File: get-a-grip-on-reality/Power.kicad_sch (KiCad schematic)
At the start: 3 parts, among them J1 Battery Connector, U1 BQ25170DSGR, U2 TLV76733DRVx

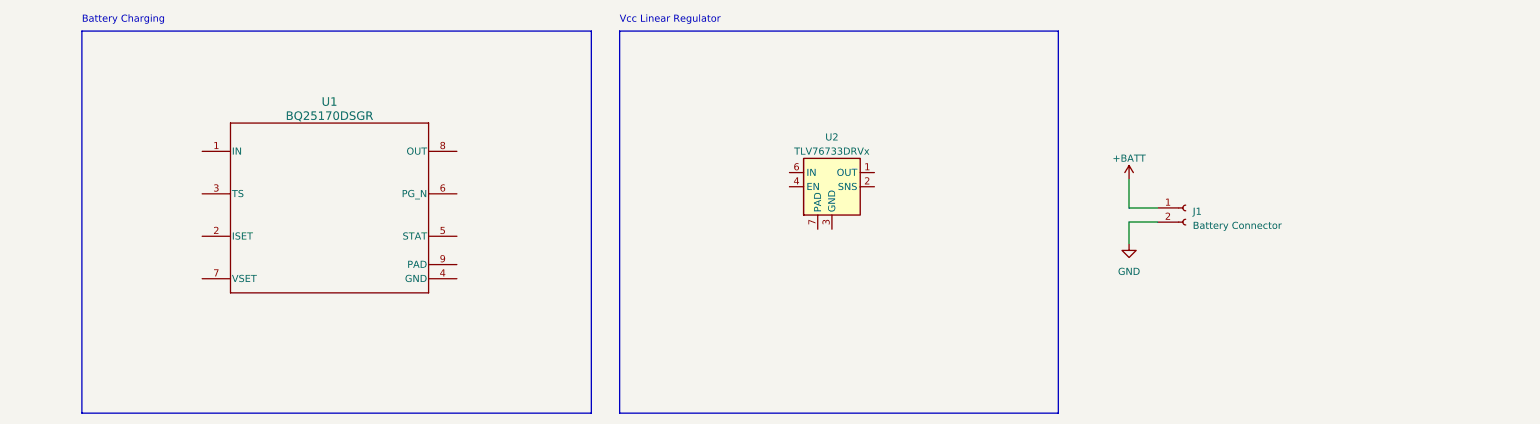
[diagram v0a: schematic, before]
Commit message: power wip
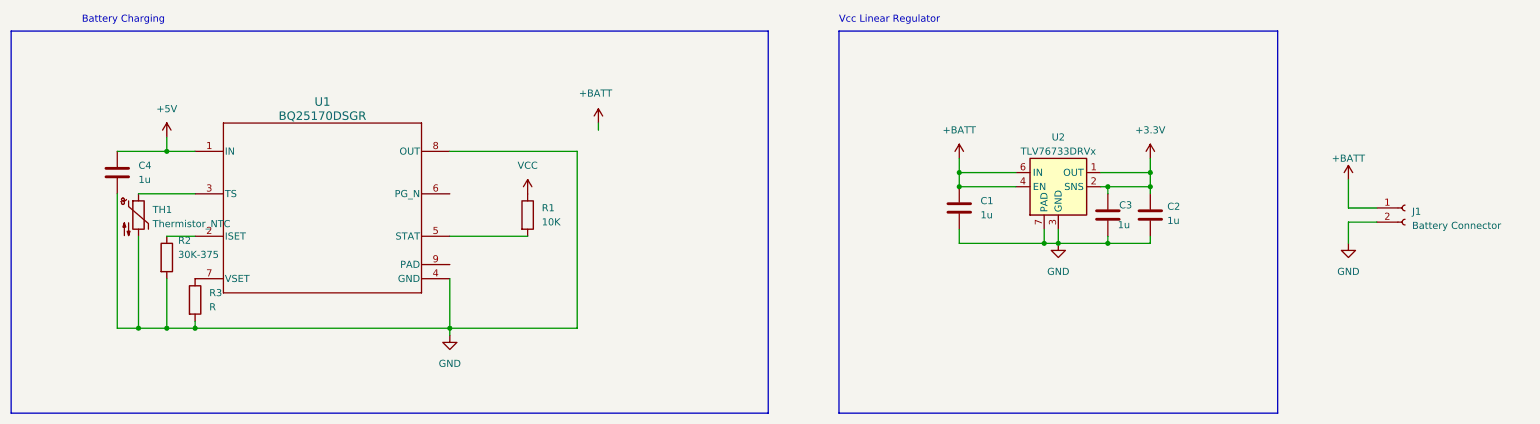
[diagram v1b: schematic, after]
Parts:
- added C1, C2, C3, C4: 1u, symbol Device:C
- added R1: 10K, symbol Device:R
- added R2: 30K-375, symbol Device:R
- added R3: R, symbol Device:R
- added TH1: Thermistor_NTC, symbol Device:Thermistor_NTC
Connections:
- net +BATT: now also U2.4 (EN), U2.6 (IN), C1.1
- net GND: now also U1.4 (GND), U1.8 (OUT), U2.3 (GND), U2.5 (GND), U2.7 (PAD), C1.2, C2.2, C3.2, C4.2, R2.2, R3.2, TH1.2
- net +3.3V: now reaches U2.1 (OUT)
- net +3.3V: now also U2.2 (SNS), C2.1, C3.1
- net +5V: now reaches U1.1 (IN)
- net +5V: now also C4.1
- net at U1.2 (ISET): now also R2.1
- net at U1.3 (TS): now also TH1.1
- net at U1.5 (STAT): now also R1.2
- net at U1.7 (VSET): now also R3.1
- new net VCC: R1.1
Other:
- moved on the sheet: J1, U1, U2
